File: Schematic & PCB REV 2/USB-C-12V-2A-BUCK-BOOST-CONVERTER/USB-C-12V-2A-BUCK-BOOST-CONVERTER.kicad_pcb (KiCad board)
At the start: 2 copper layers, 55.2 x 26.7 mm, 30 parts, among them J1 Conn_01x02_Pin, U3 TPS61089RNRR

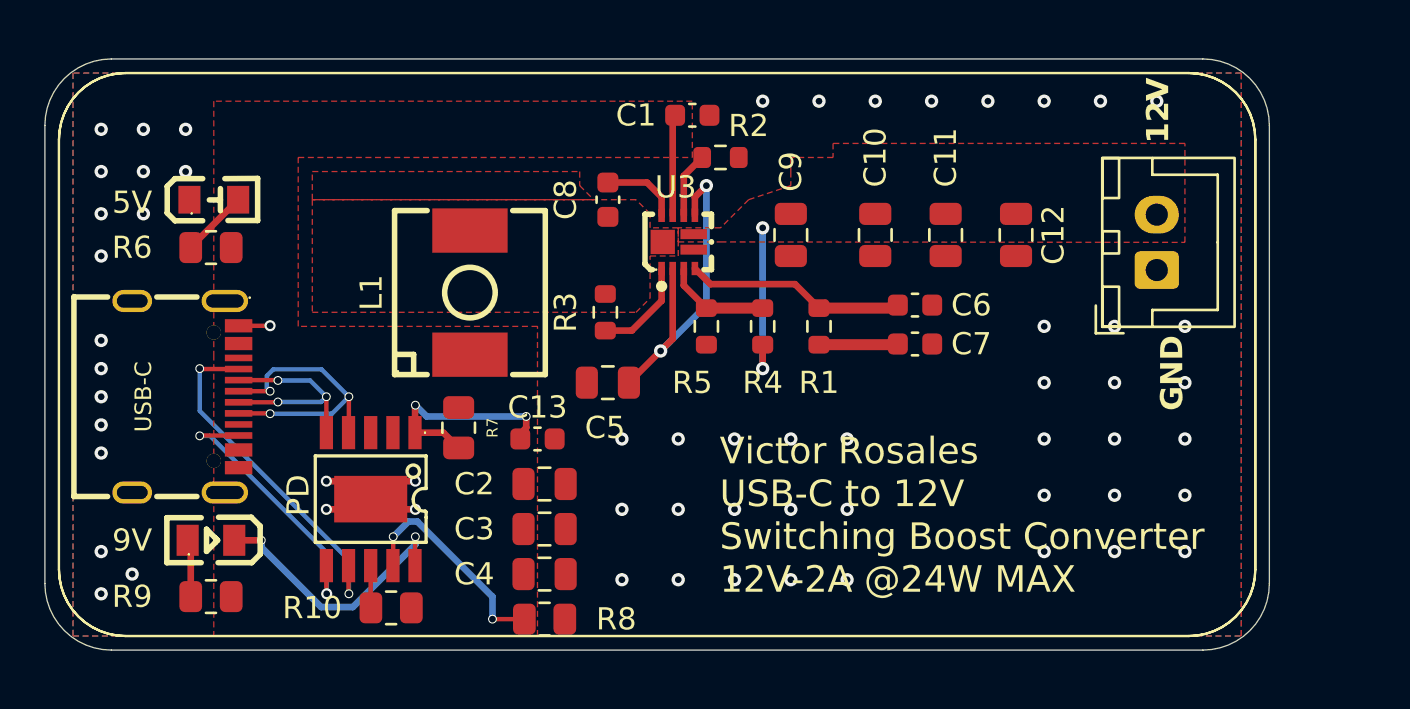
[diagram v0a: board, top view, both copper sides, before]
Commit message: Rev finished board
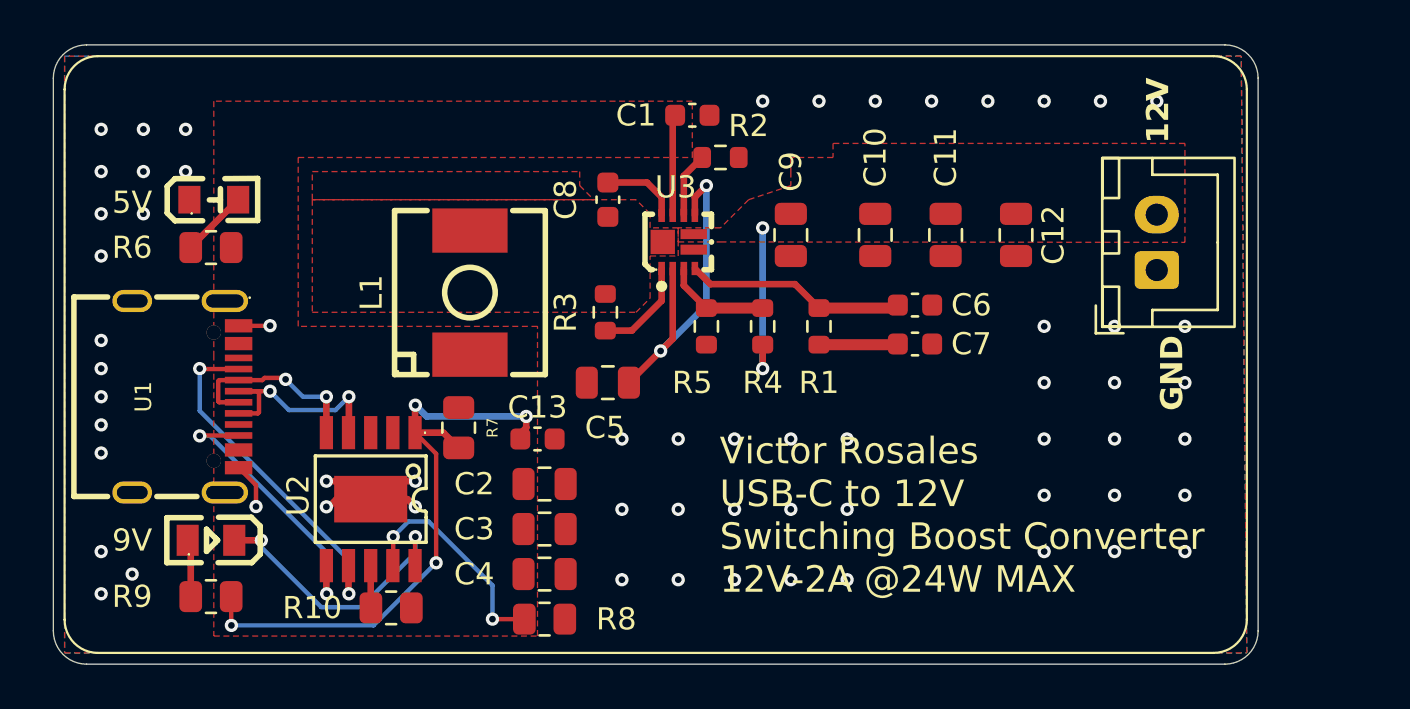
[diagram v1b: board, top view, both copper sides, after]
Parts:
- renumbered USB-C to U1, PD to U2
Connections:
- net Net-(J1-Pin_2) renamed +12V
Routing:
- net VDD: track 9.84 -> 27.9 mm, vias 2 -> 4
- net DP: track 13.4 -> 10.2 mm, vias 3 -> 2
- net GND: track 10.7 -> 12.8 mm, vias 60 -> 61
- net DM: track 9.97 -> 8.93 mm, vias 3 -> 2
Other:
- board size 55.2 x 26.7 mm -> 54.4 x 27.9 mm
